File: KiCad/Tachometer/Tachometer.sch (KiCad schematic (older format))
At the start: 108 parts, among them J1 PJ301M-12, J2 PJ301M-12, J3 PJ301M-12, J4 PJ301M-12, J5 PJ301M-12, J6 PJ301M-12, J7 PJ301M-12, J8 PJ301M-12, J9 PJ301M-12, Q1 2N3904, Q10 2N3904, Q11 2N3904, Q12 2N3904, Q13 2N3904, Q14 2N3904, Q15 2N3904, Q16 2N3904, Q17 2N3904, Q18 2N3904, Q2 2N3904, Q3 2N3904, Q4 2N3904, Q5 2N3904, Q6 2N3904, Q7 2N3904, Q8 2N3904, Q9 2N3904

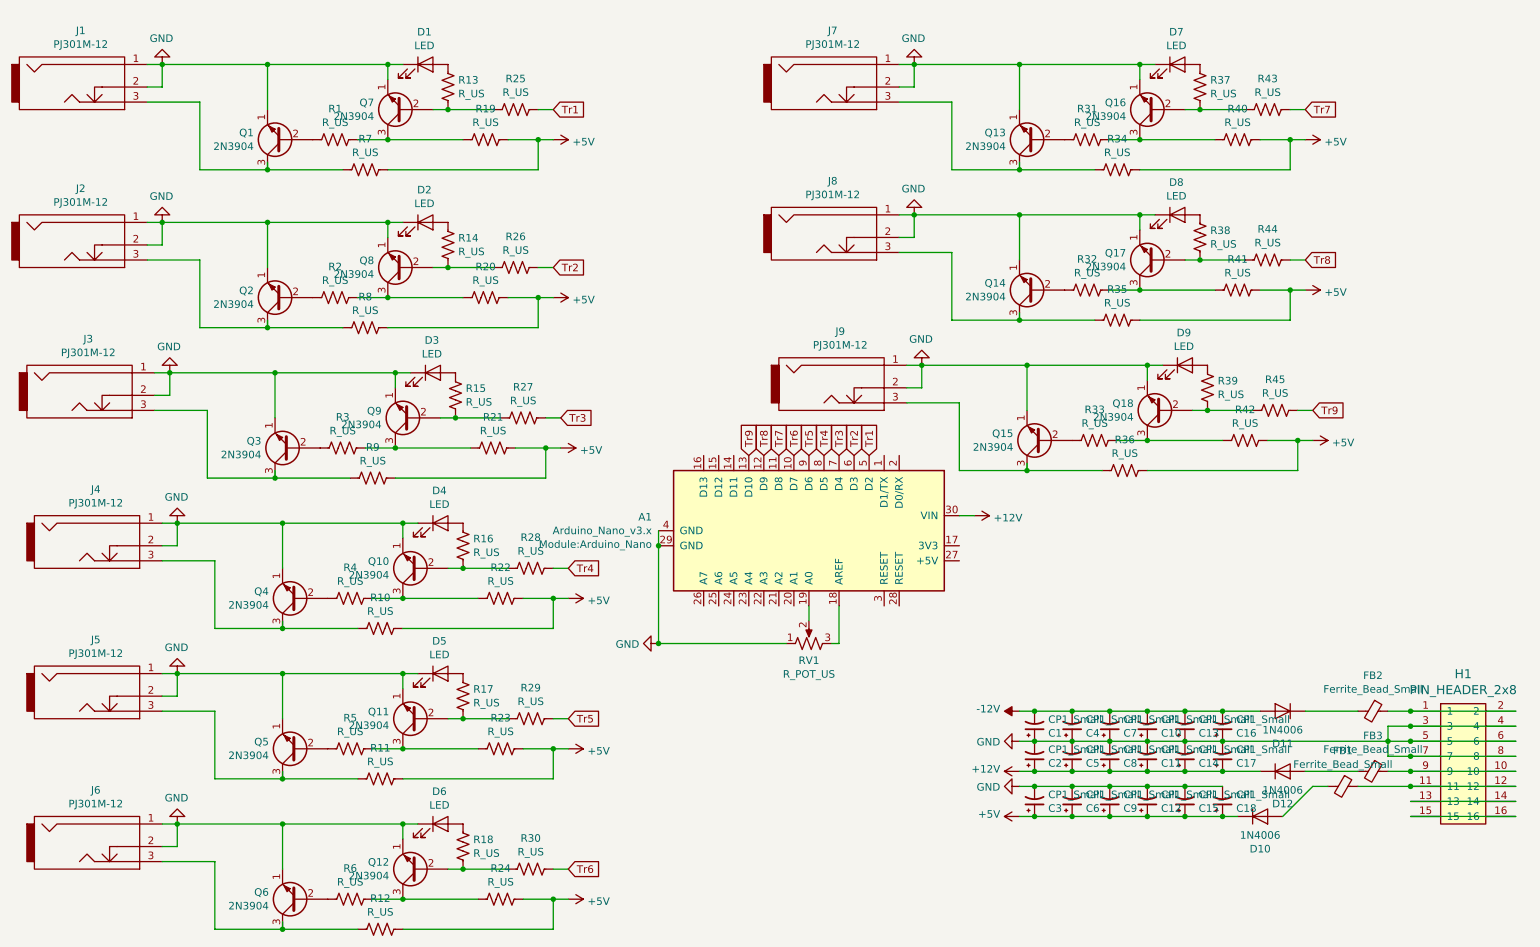
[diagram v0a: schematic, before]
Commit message: all work
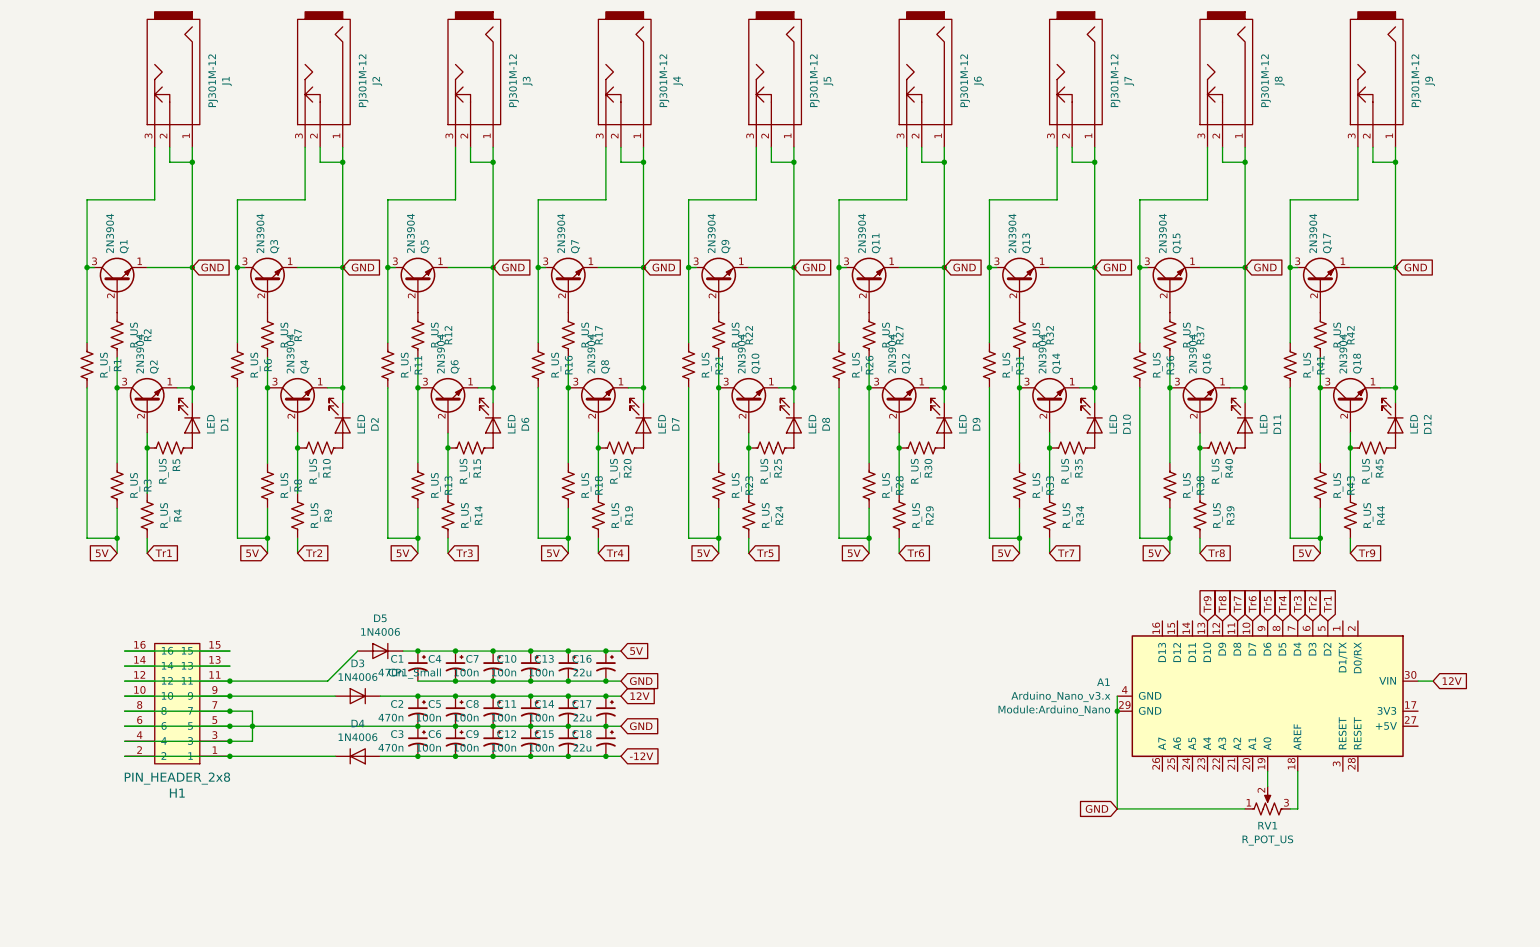
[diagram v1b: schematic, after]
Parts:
- removed FB1, FB2, FB3: Ferrite_Bead_Small, symbol Device:Ferrite_Bead_Small
- C1: renamed from C18; value CP1_Small -> 470n
- C10: renamed from C9; value CP1_Small -> 100n
- C11: renamed from C8; value CP1_Small -> 100n
- C12: renamed from C7; value CP1_Small -> 100n
- C13: renamed from C6; value CP1_Small -> 100n
- C14: renamed from C5; value CP1_Small -> 100n
- C15: renamed from C4; value CP1_Small -> 100n
- C16: renamed from C3; value CP1_Small -> 22u
- C17: renamed from C2; value CP1_Small -> 22u
- C18: renamed from C1; value CP1_Small -> 22u
- C2: renamed from C17; value CP1_Small -> 470n
- C3: renamed from C16; value CP1_Small -> 470n
- C5: renamed from C14; value CP1_Small -> 100n
- C6: renamed from C13; value CP1_Small -> 100n
- C7: renamed from C12; value CP1_Small -> 100n
- C8: renamed from C11; value CP1_Small -> 100n
- C9: renamed from C10; value CP1_Small -> 100n
- renumbered C15 to C4, D6 to D1, D9 to D10, D8 to D11, D7 to D12, D5 to D2, D12 to D3, D11 to D4, D10 to D5, D4 to D6, D3 to D7, D2 to D8, D1 to D9, J6 to J1, J5 to J2, J4 to J3, J3 to J4, J2 to J5, J1 to J6, J9 to J7, J7 to J9, Q6 to Q1, Q8 to Q10, Q1 to Q11, Q7 to Q12, Q15 to Q13, Q18 to Q14, Q14 to Q15, Q17 to Q16, Q13 to Q17, Q16 to Q18, Q12 to Q2, Q5 to Q3, Q11 to Q4, Q4 to Q5, Q10 to Q6, Q3 to Q7, Q9 to Q8, Q2 to Q9, R12 to R1, R17 to R10, R10 to R11, R4 to R12, R22 to R13, R28 to R14, R16 to R15, R9 to R16, R3 to R17, R21 to R18, R27 to R19, R6 to R2, R15 to R20, R8 to R21, R2 to R22, R20 to R23, R26 to R24, R14 to R25, R7 to R26, R1 to R27, R19 to R28, R25 to R29, R24 to R3, R13 to R30, R36 to R31, R33 to R32, R42 to R33, R45 to R34, R39 to R35, R35 to R36, R32 to R37, R41 to R38, R44 to R39, R30 to R4, R38 to R40, R34 to R41, R31 to R42, R40 to R43, R43 to R44, R37 to R45, R18 to R5, R11 to R6, R5 to R7, R23 to R8, R29 to R9
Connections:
- net labels added: 12V, 5V
- net labels removed: +12V, +5V
- wire segments 259 -> 256
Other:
- moved on the sheet: A1, C1, C10, C11, C12, C13, C14, C15, C16, C17, C18, C2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
